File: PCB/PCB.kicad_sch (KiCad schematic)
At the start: 12 parts, among them U1 Buck Converter Module, U2 Ultrasonic Sensor, U3 ESP32-WROOM-32

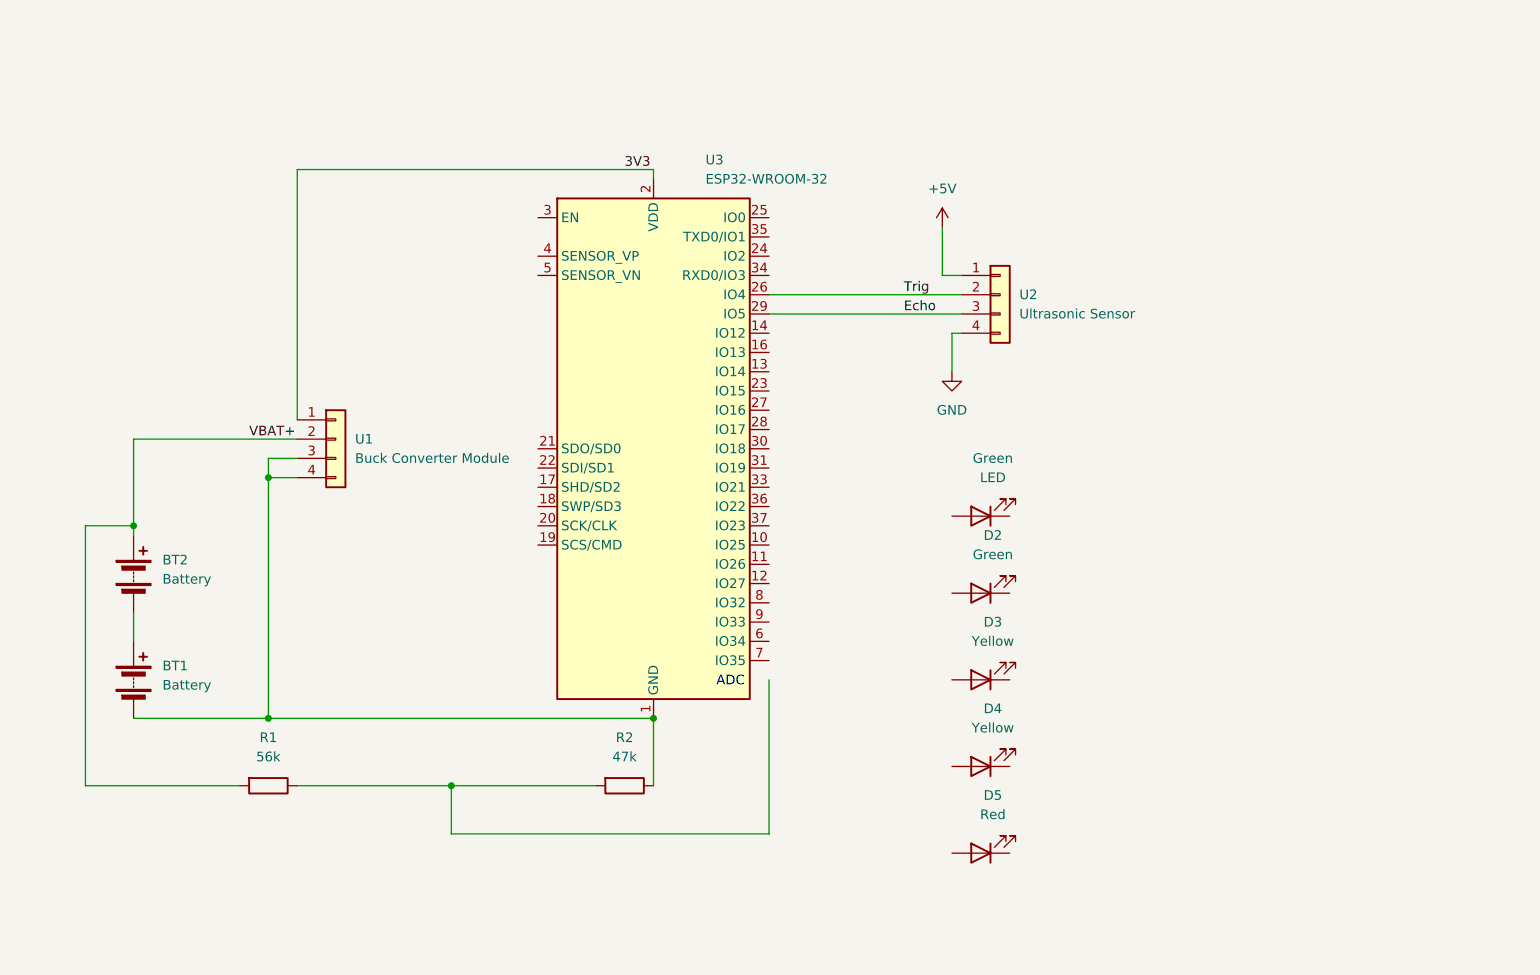
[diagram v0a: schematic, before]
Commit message: Update PCB.kicad_sch
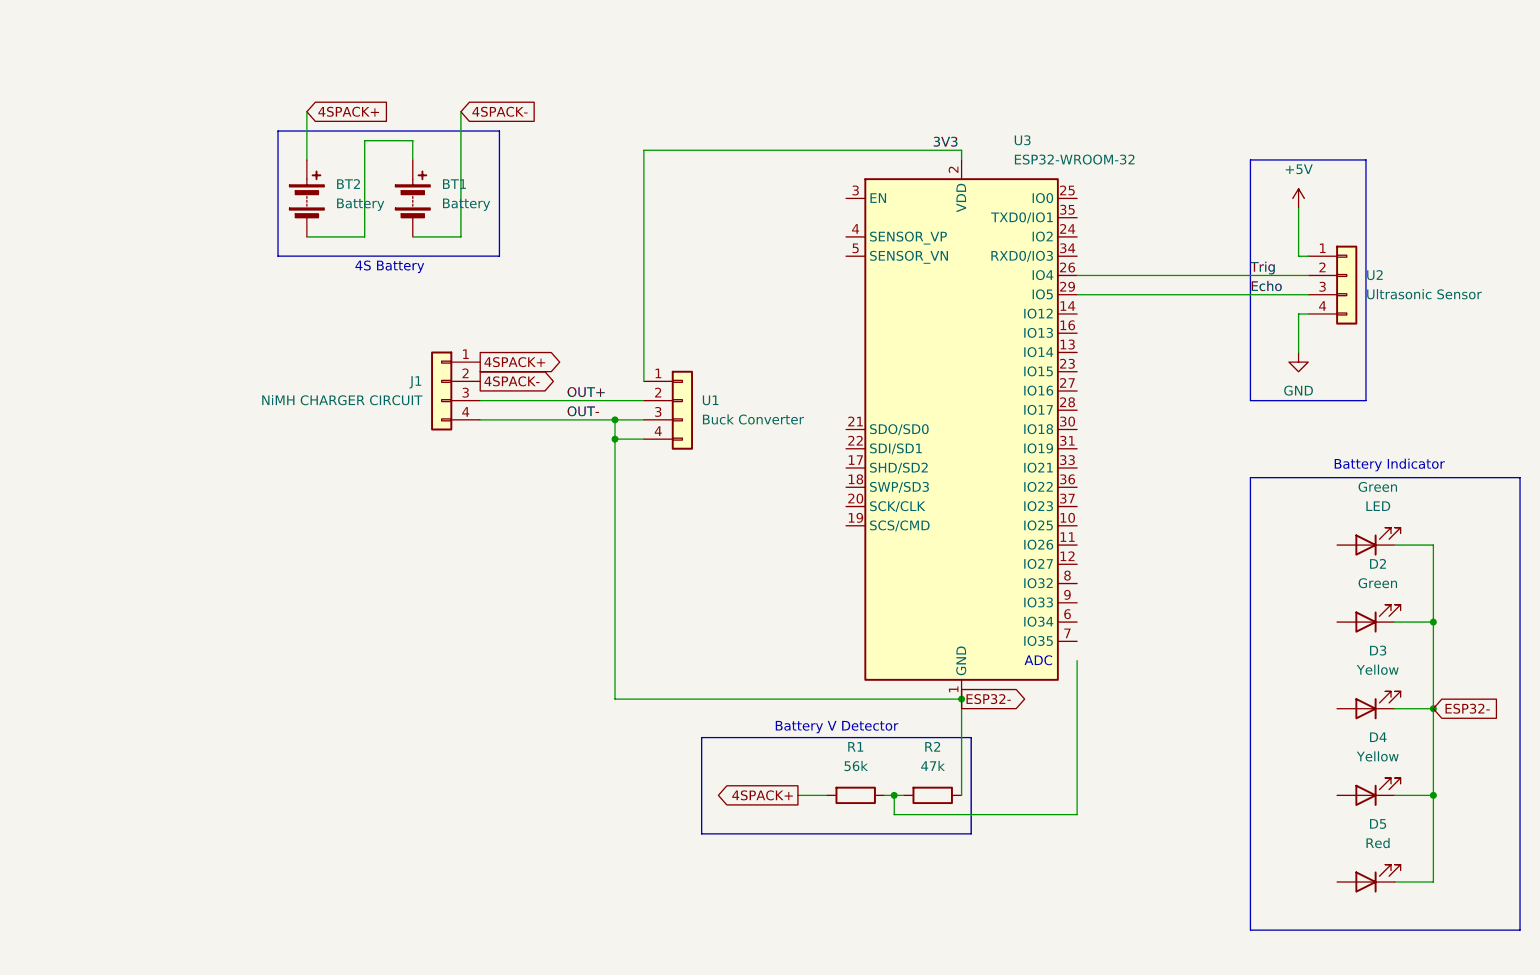
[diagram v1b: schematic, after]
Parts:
- added J1: NiMH CHARGER CIRCUIT, symbol Connector_Generic:Conn_01x04
- U1: value Buck Converter Module -> Buck Converter
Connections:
- net ESP32-: now reaches R2.1, U1.3 (Pin_3), U1.4 (Pin_4), U3.1 (GND), U3.15 (GND), U3.38 (GND), U3.39 (GND)
- net ESP32-: now also D2.1 (K), D3.1 (K), D4.1 (K), D5.1 (K), Green.1 (K), J1.4 (Pin_4); no longer BT1.2 (-)
- net VBAT+ renamed 4SPACK+
- net 4SPACK+: now also J1.1 (Pin_1); no longer U1.2 (Pin_2)
- new net 4SPACK-: BT1.2 (-), J1.2 (Pin_2)
- new net OUT+: J1.3 (Pin_3), U1.2 (Pin_2)
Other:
- note added: "4S Battery"
- note added: "Battery Indicator"
- note added: "Battery V Detector"
- moved on the sheet: BT1, BT2, D2, D3, D4, D5, Green, R1, R2, U1, U2, U3

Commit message: Update PCB.kicad_sch
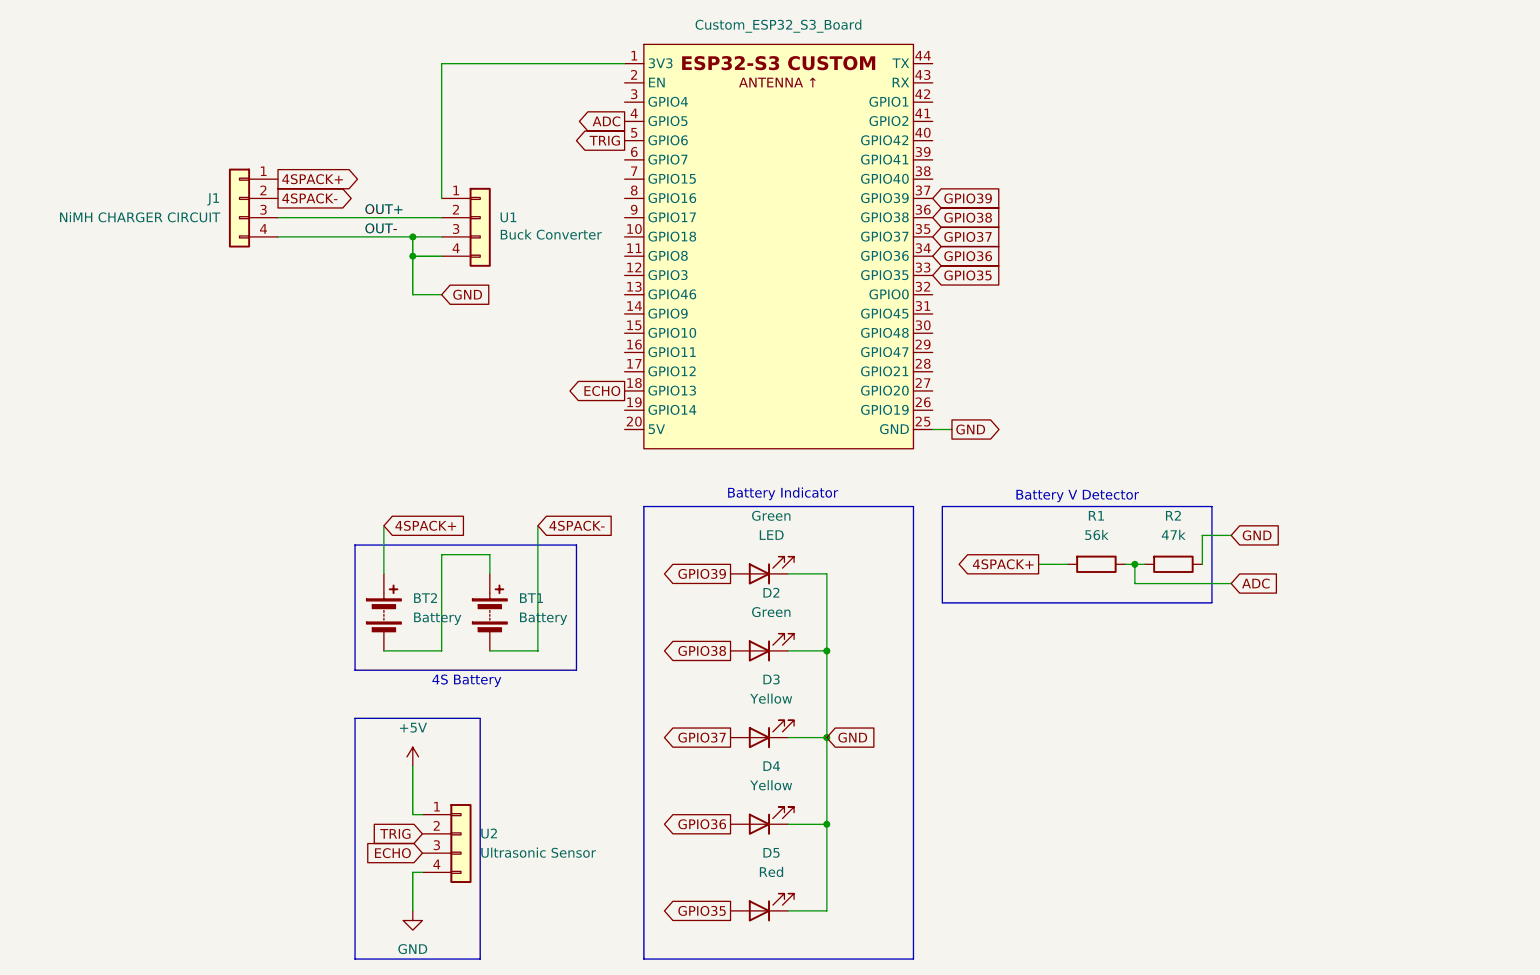
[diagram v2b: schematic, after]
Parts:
- removed U3: ESP32-WROOM-32, RF_Module:ESP32-WROOM-32, symbol RF_Module:ESP32-WROOM-32
- added U4: Custom_ESP32_S3_Board, symbol ESP32_S3_Board:Custom_ESP32_S3_Board
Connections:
- net ESP32- is gone; now on net GND: D2.1 (K), D3.1 (K), D4.1 (K), D5.1 (K), Green.1 (K), J1.4 (Pin_4), R2.1, U1.3 (Pin_3), U1.4 (Pin_4)
- net GND: now also U4.25 (GND)
- net GPIO38: now reaches D2.2 (A)
- net GPIO38: now also U4.36 (GPIO38)
- net GPIO37: now reaches D3.2 (A)
- net GPIO37: now also U4.35 (GPIO37)
- net GPIO36: now reaches D4.2 (A)
- net GPIO36: now also U4.34 (GPIO36)
- net ADC: now reaches R1.1, R2.2
- net ADC: now also U4.4 (GPIO5)
- net GPIO35: now reaches D5.2 (A)
- net GPIO35: now also U4.33 (GPIO35)
- net GPIO39: now reaches Green.2 (A)
- net GPIO39: now also U4.37 (GPIO39)
- net 3V3: no longer names the net of U1.1 (Pin_1)
- net 3V3: now also U4.1 (3V3)
- net Echo renamed ECHO
- net ECHO: now also U4.18 (GPIO13)
- net Trig renamed TRIG
- net TRIG: now also U4.5 (GPIO6)
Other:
- note removed: "ADC"
- moved on the sheet: BT1, BT2, D2, D3, D4, D5, Green, J1, R1, R2, U1, U2
